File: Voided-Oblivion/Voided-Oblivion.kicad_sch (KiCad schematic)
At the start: 131 parts, among them J1 Top male, J10 Sub-Module TL, J11 Sub-Module LT, J12 Sub-Module TR, J16 Sub-Module BL, J17 Sub-Module LB, J18 Sub-Module BR, J19 Sub-Module RB, J2 Top female, J20 Sub-Module RT, J3 Right male, J4 Right female, J5 Left male, J6 Left female, J7 Bottom male, J8 Bottom female, J9 SM03B-SRSS-TB, SW1 boot, SW2 reset, U1 RP2350_80QFN, U3 W25Q128JVS, U4 W25Q128JVS, Y1 ABM8-272-T3

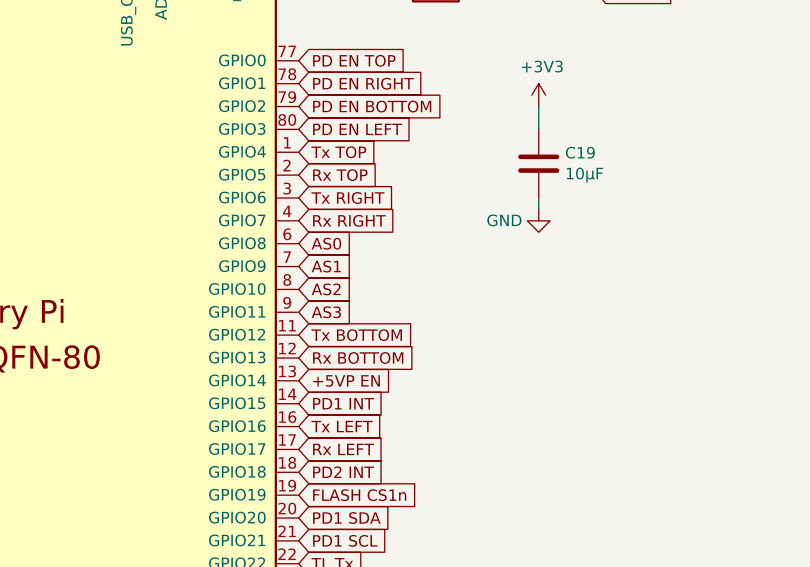
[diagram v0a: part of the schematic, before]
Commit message: still cis tho
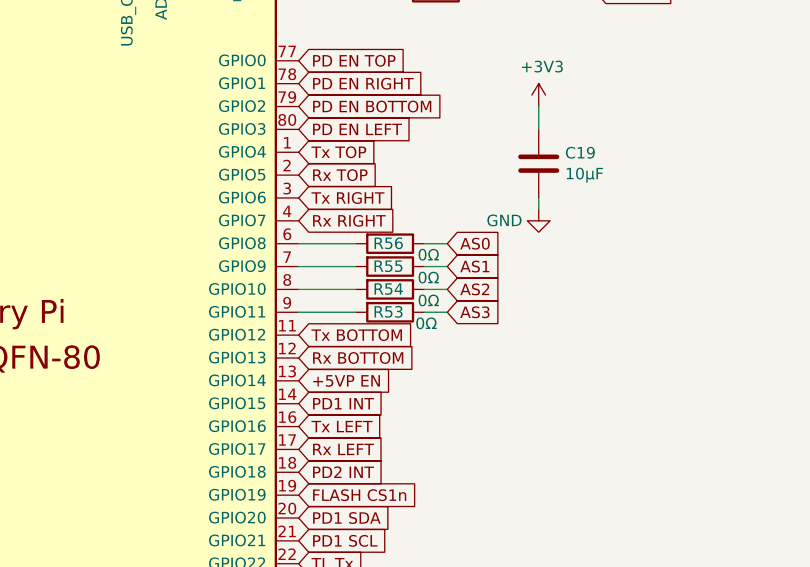
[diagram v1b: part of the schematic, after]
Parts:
- added R53, R54, R55, R56: 0Ω, Resistor_SMD:R_0402_1005Metric, symbol Device:R
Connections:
- net AS0: now also R56.1; no longer U1.6 (GPIO8)
- net AS1: now also R55.1; no longer U1.7 (GPIO9)
- net AS2: now also R54.1; no longer U1.8 (GPIO10)
- net AS3: now also R53.1; no longer U1.9 (GPIO11)
- new net: R56.2, U1.6 (GPIO8)
- new net: R55.2, U1.7 (GPIO9)
- new net: R53.2, U1.9 (GPIO11)
- new net: R54.2, U1.8 (GPIO10)
